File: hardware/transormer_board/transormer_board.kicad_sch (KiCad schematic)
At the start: 6 parts, among them J1 orange, J2 black, J3 PE, J4 Conn_02x04_Top_Bottom, J5 red, J6 grey

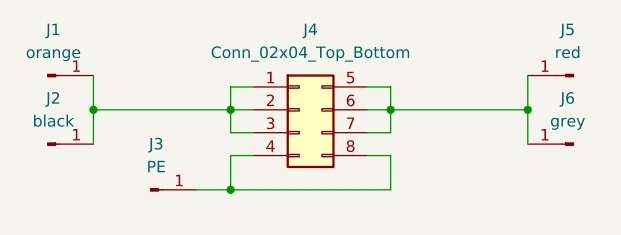
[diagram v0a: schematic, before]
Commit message: update some shit
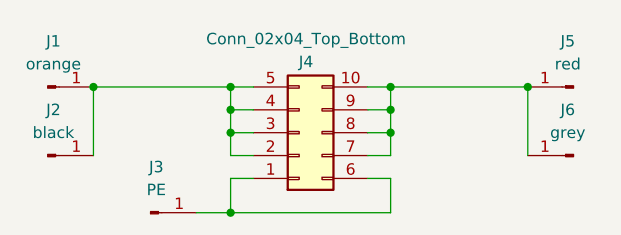
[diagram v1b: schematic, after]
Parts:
- J4: footprint Connector_Molex:Molex_Mini-Fit_Jr_5566-08A_2x04_P4.20mm_Vertical -> Connector_Molex:Molex_Nano-Fit_105310-xx10_2x05_P2.50mm_Vertical; symbol Connector_Generic:Conn_02x04_Top_Bottom -> Connector_Generic:Conn_02x05_Top_Bottom
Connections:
- net at J1.1 (Pin_1), J2.1 (Pin_1), J4.2 (Pin_2)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: now also J4.4 (Pin_4), J4.5 (Pin_5); no longer J4.1 (Pin_1)
- net at J4.7 (Pin_7), J5.1 (Pin_1), J6.1 (Pin_1): now also J4.10 (Pin_10), J4.8 (Pin_8), J4.9 (Pin_9); no longer J4.5 (Pin_5), J4.6 (Pin_6)
- new net: J3.1 (Pin_1), J4.1 (Pin_1), J4.6 (Pin_6)
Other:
- moved on the sheet: J1, J2, J3, J5, J6

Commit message: save work
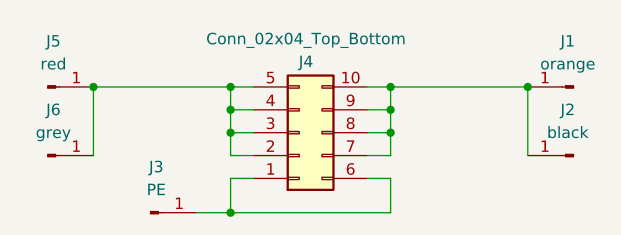
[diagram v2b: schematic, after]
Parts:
- J4: footprint Connector_Molex:Molex_Nano-Fit_105310-xx10_2x05_P2.50mm_Vertical -> Connector_Molex:Molex_Micro-Fit_3.0_43045-1012_2x05_P3.00mm_Vertical
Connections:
- net at J4.2 (Pin_2), J4.3 (Pin_3), J4.4 (Pin_4)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: now also J5.1 (Pin_1), J6.1 (Pin_1); no longer J1.1 (Pin_1), J2.1 (Pin_1)
- net at J4.10 (Pin_10), J4.7 (Pin_7), J4.8 (Pin_8)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: now also J1.1 (Pin_1), J2.1 (Pin_1); no longer J5.1 (Pin_1), J6.1 (Pin_1)
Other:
- moved on the sheet: J1, J2, J5, J6
